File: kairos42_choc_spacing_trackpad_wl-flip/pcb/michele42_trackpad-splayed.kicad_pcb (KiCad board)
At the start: 2 copper layers, 139.6 x 90.1 mm, 108 parts, among them J1 Battery, J2 OLED-5Pin, J4 LED, SW1 SW_Power, U1 MCU_Nice_Nano_V2

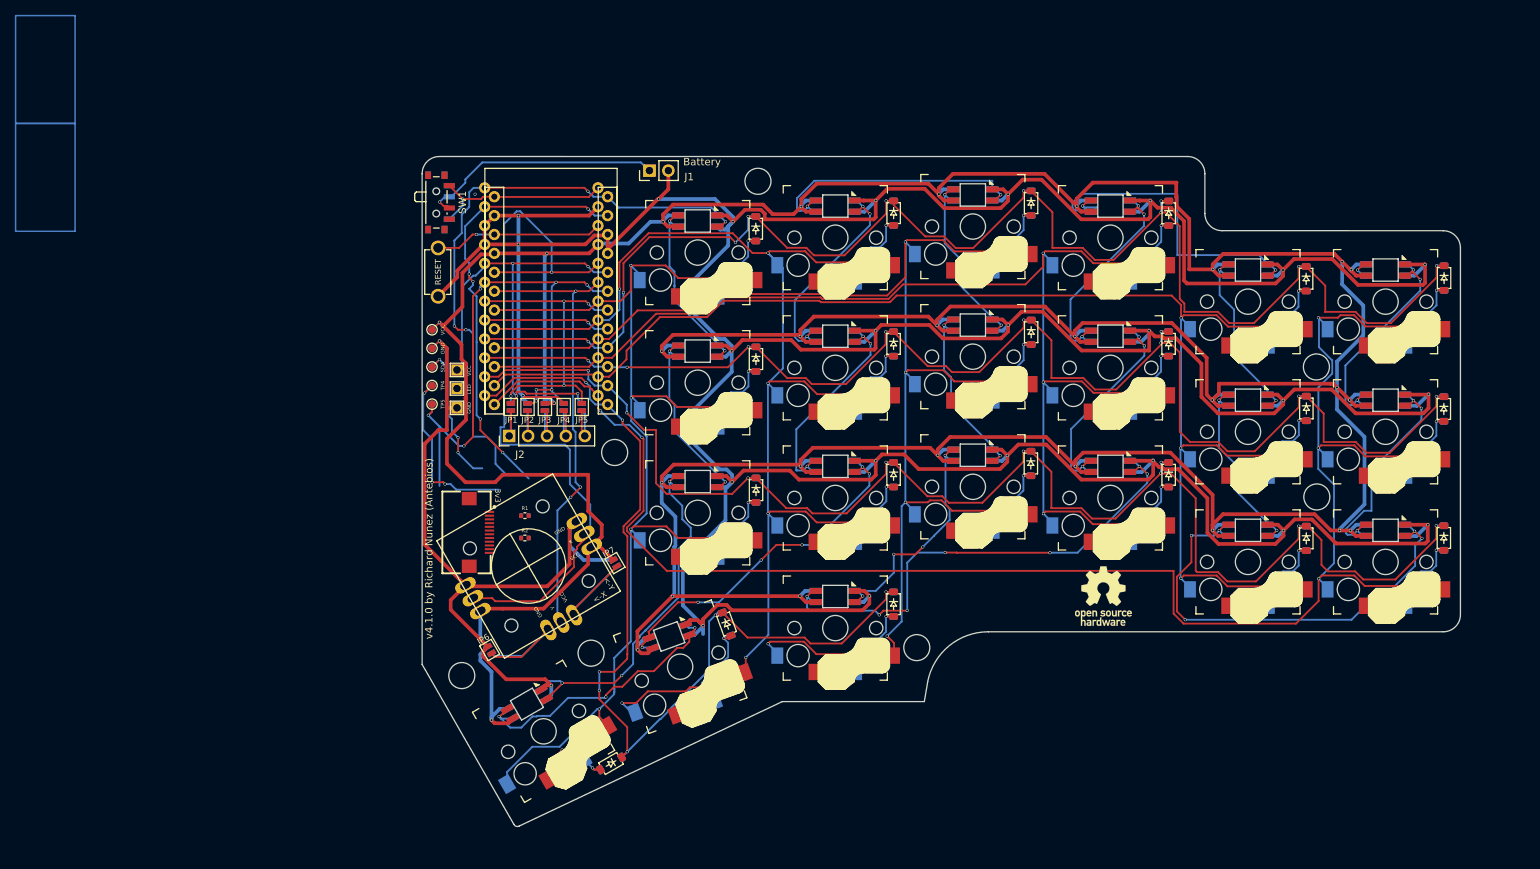
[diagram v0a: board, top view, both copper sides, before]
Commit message: Trackpad cas stuff - wip again
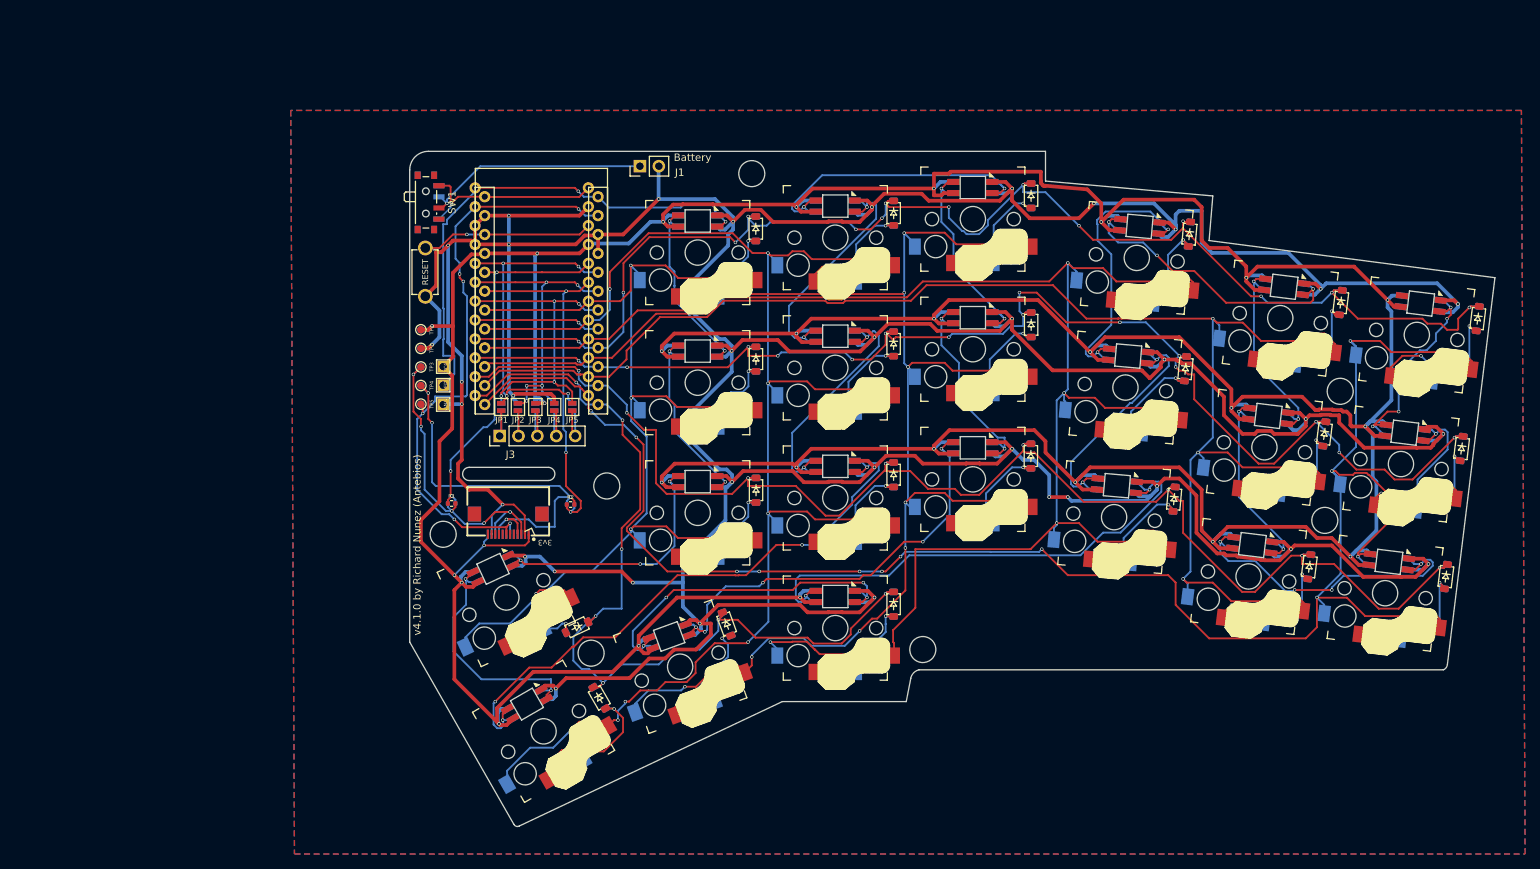
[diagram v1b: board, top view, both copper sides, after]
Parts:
- removed GND, SDA, VCC: TestPoint, TestPoint:TestPoint_Pad_D1.0mm
- removed JP6 (x2), JP7 (x2): Jumper, mylocal_footprints:jumper_data-MOD
- removed REF** (x2): OSHW-Logo_7.5x8mm_SilkScreen, Symbol:OSHW-Logo_7.5x8mm_SilkScreen
- removed Thumbstick1: ~, mylocal_footprints:Mini 2-Axis Analog Thumbstick
- added D26: Diode, mylocal_footprints:Diode_SOD-123-double-sided, F.Cu at (89.0, 120.0)
- added D4: SK6812MINI-E, mylocal_footprints:SK6812-MINI-E-double-side, F.Cu at (77.7, 112.1)
- added J3: ~, vik:vik-keyboard-connector-horizontal, B.Cu at (79.8, 105.5)
- added S4: Keyswitch, mylocal_footprints:Choc_Hotswap-double-sided, F.Cu at (79.5, 116.0)
- added TP1: TestPoint, TestPoint:TestPoint_Pad_D1.0mm, B.Cu at (68.0, 80.0)
- added TP2: TestPoint, TestPoint:TestPoint_Pad_D1.0mm, B.Cu at (68.0, 82.5)
- added TP3: TestPoint, TestPoint:TestPoint_Pad_D1.0mm, F.Cu at (68.0, 85.0)
- TP1, TP2: moved to F.Cu
- moved H6 19.2 mm to (71.0, 107.5)
- moved R1 9.99 mm to (72.1, 103.4) (x2)
- moved D30 8.96 mm to (92.0, 129.5), turned to -60 degrees
- moved R2 7.62 mm to (88.1, 103.5) (x2)
- moved D42 7.09 mm to (210.1, 78.5), turned to -97 degrees
- moved D20 6.52 mm to (202.5, 76.5), turned to -7 degrees
- moved S20 6.14 mm to (201.9, 80.7), turned to 173 degrees
- moved D43 5.83 mm to (208.0, 96.0), turned to -97 degrees
- moved D39 5.65 mm to (191.7, 76.3), turned to -97 degrees
- moved D17 5.35 mm to (184.1, 74.2), turned to -7 degrees
- moved D44 5.20 mm to (205.8, 113.2), turned to -97 degrees
- moved D21 5.08 mm to (200.3, 93.8), turned to -7 degrees
- moved J2 4.90 mm to (79.8, 105.5), turned to 180 degrees
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- renumbered D22 to D1, D30 to D10, D36 to D11, D41 to D12, D25 to D13, D31 to D14, D37 to D15, D42 to D16, D26 to D17, D32 to D18, D38 to D19, D28 to D2, D27 to D20, D33 to D21, D39 to D22, D1 to D23, D7 to D24, D13 to D25, D2 to D27, D8 to D28, D14 to D29, D34 to D3, D19 to D30, D3 to D31, D9 to D32, D15 to D33, D20 to D34, D4 to D35, D10 to D36, D16 to D37, D21 to D38, D5 to D39, D11 to D40, D17 to D41, D6 to D42, D12 to D43, D18 to D44, D23 to D5, D29 to D6, D35 to D7, D40 to D8, D24 to D9, J3 to J2, J2 to J3, S9 to S10, S15 to S11, S20 to S12, S4 to S13, S10 to S14, S16 to S15, S21 to S16, S5 to S17, S11 to S18, S17 to S19, S7 to S2, S6 to S20, S12 to S21, S18 to S22, S13 to S3, S2 to S5, S8 to S6, S14 to S7, S19 to S8, S3 to S9
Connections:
- D11 pad 2: Net-(D36-DOUT) -> Net-(D11-DOUT)
- D12 pad 2: Net-(D35-DIN) -> Net-(D12-DOUT)
- D12 pad 4: Net-(D40-DOUT) -> Net-(D11-DOUT)
- D16 pad 4: Net-(D36-DOUT) -> Net-(D12-DOUT)
- D17 pad 3: Net-(D26-GND) -> GND
- D18 pad 3: Net-(D26-GND) -> GND
- D19 pad 3: Net-(D26-GND) -> GND
- D20 pad 3: Net-(D26-GND) -> GND
- D21 pad 3: Net-(D26-GND) -> GND
- D22 pad 3: Net-(D26-GND) -> GND
- D3 pad 2: Net-(D34-DOUT) -> Net-(D3-DOUT)
- D7 pad 4: Net-(D35-DIN) -> Net-(D7-DIN)
- D8 pad 2: Net-(D40-DOUT) -> Net-(D7-DIN)
- D8 pad 4: Net-(D34-DOUT) -> Net-(D4-DOUT)
- S12 pad 2: Column 1 -> Column 2
- S16 pad 2: Column 2 -> Column 3
- S8 pad 2: Column 0 -> Column 1
- U1 pad 1: SDA -> LED
- U1 pad 19: ThumbY -> SCL
- U1 pad 2: SCL -> DRDY
- U1 pad 20: ThumbX -> SDA
- U1 pad 5: LED -> MOSI
- U1 pad 6: DRDY -> SCK
- U1 pad 7: unconnected-(U1-D4-Pad7) -> CS
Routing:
- net ThumbX: track 100.6 -> 0.00 mm, vias 1 -> 0
- net Net-(D7-DIN): track 0.00 -> 80.5 mm, vias 0 -> 4
- net ThumbY: track 61.2 -> 0.00 mm, vias 3 -> 0
- net Column 3: track 180.6 -> 240.6 mm, vias 3 -> 4
- net Net-(D11-DOUT): track 0.00 -> 59.0 mm, vias 0 -> 5
- net Net-(D34-DOUT): track 49.3 -> 0.00 mm, vias 3 -> 0
- net Net-(D35-DIN): track 47.5 -> 0.00 mm, vias 6 -> 0
- net Net-(D12-DOUT): track 0.00 -> 46.6 mm, vias 0 -> 4
- net DRDY: track 41.1 -> 82.0 mm, vias 3 -> 6
- net Net-(D40-DOUT): track 38.3 -> 0.00 mm, vias 3 -> 0
- net Net-(D3-DOUT): track 0.00 -> 37.1 mm, vias 0 -> 3
- net Net-(D4-DOUT): track 0.00 -> 32.7 mm, vias 0 -> 2
- net Net-(D36-DOUT): track 32.0 -> 0.00 mm, vias 4 -> 0
- net TP-SCL: track 24.8 -> 55.3 mm, vias 3 -> 4
- net TP-SDA: track 17.7 -> 43.3 mm, vias 3 -> 5
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- added copper zone on B.Cu, net (none)
- added copper zone on F.Cu, net (none)
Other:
- board size 139.6 x 90.1 mm -> 145.9 x 90.8 mm
